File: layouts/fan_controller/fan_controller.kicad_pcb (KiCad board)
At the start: 2 copper layers, 6 parts

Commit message: Add MCU as build target
use this ato branch to fix build:
https://github.com/atopile/atopile/pull/979
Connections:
- D1 pad 2: gnd-2 -> gnd-1
- FanConnector1 pad 1: gnd-2 -> gnd-1
- Q1 pad 2: gnd-2 -> gnd-1
- Q1 pad 3: gnd -> gnd-2
- R1 pad 2: gnd-1 -> gnd
- R2 pad 2: gnd-2 -> gnd-1
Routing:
- net gnd-2: track 6.53 -> 0.00 mm
- net gnd-1: track 0.00 -> 6.53 mm

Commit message: Migrate layout partially
omit routing and zones amongst others
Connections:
- D1 pad 2: gnd-1 -> gnd
- FanConnector1 pad 1: gnd-1 -> gnd
- Q1 pad 2: gnd-1 -> gnd
- Q1 pad 3: gnd-2 -> gnd-1
- R1 pad 2: gnd -> gnd-2
- R2 pad 2: gnd-1 -> gnd
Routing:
- net gnd-1: track 6.53 -> 0.00 mm
- net gnd: track 0.00 -> 6.53 mm
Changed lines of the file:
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@@
             (outputdirectory "")))
     (net 0 "")
-    (net 1 "gnd-1")
-    (net 2 "gnd-2")
+    (net 1 "gnd")
+    (net 2 "gnd-1")
     (net 3 "cathode")
     (net 4 "fan_connector.footprint.pins[3].net-net")
     (net 5 "hv")
-    (net 6 "gnd")
+    (net 6 "gnd-2")
     (net 7 "line")
     (net 8 "fan_connector.footprint.pins[2].net-net")
@@
             (layers "F.Cu" "F.Paste" "F.Mask")
             (remove_unused_layers no)
-            (net 1 "gnd-1")))
+            (net 1 "gnd")))
     (footprint "atopile:SOT-23-3_L2.9-W1.3-P1.90-LS2.4-BL-1-fcaf94"
         (layer "F.Cu")
@@
             (layers "F.Cu" "F.Paste" "F.Mask")
             (remove_unused_layers no)
-            (net 1 "gnd-1"))
+            (net 1 "gnd"))
         (pad "3" smd rect
             (at 0 -1 0)
@@
             (layers "F.Cu" "F.Paste" "F.Mask")
             (remove_unused_layers no)
-            (net 2 "gnd-2")))
+            (net 2 "gnd-1")))
     (footprint "atopile:R0603-ebcab9"
         (layer "F.Cu")
@@
             (layers "F.Cu" "F.Paste" "F.Mask")
             (remove_unused_layers no)
-            (net 6 "gnd")))
+            (net 6 "gnd-2")))
     (footprint "atopile:CONN-SMD_1.25-2P-ea2134"
         (layer "F.Cu")
@@
             (layers "F.Cu" "F.Paste" "F.Mask")
             (remove_unused_layers no)
-            (net 1 "gnd-1"))
+            (net 1 "gnd"))
         (pad "2" smd rect
             (at 0.63 -1.45 90)
@@
             (layers "F.Cu" "F.Paste" "F.Mask")
             (remove_unused_layers no)
-            (net 1 "gnd-1")))
+            (net 1 "gnd")))
     (segment
         (start 10.83 -4.5)

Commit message: Update layouts
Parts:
- D2: value infV -> (none)
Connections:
- Q1 pad 3: gnd-1 -> gnd-2
- R1 pad 2: gnd-2 -> gnd-1

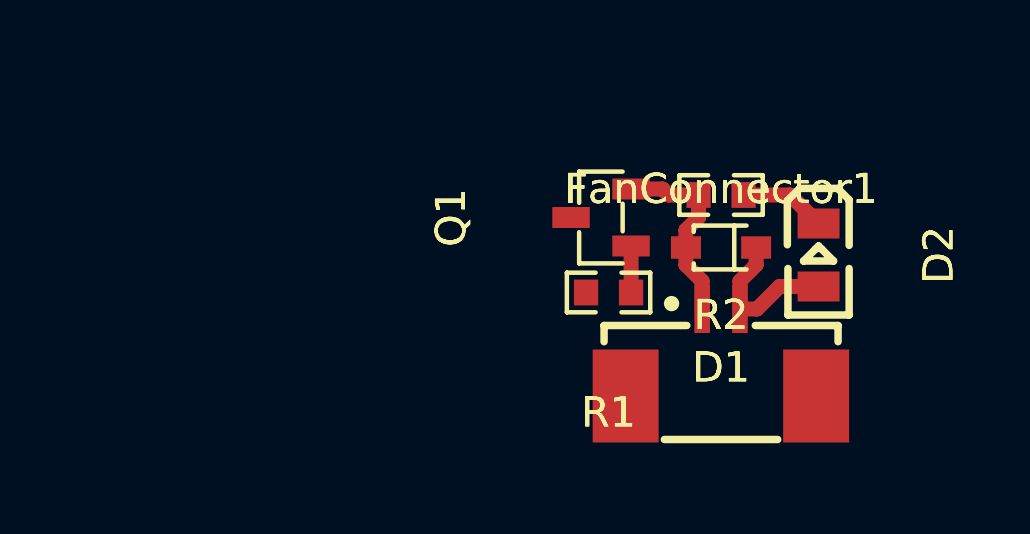
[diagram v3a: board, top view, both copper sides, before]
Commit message: Update layout
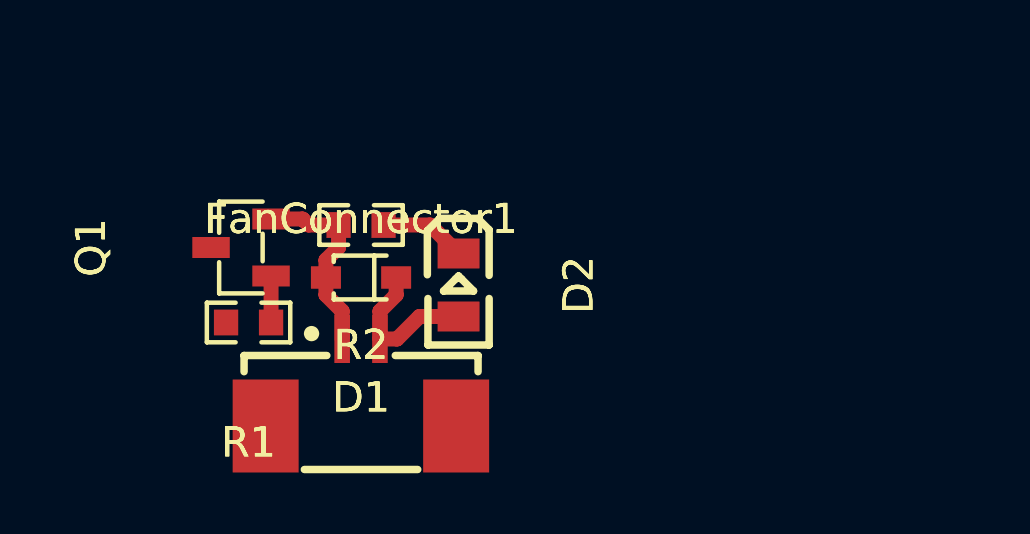
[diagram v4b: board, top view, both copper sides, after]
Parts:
- moved D1 12.0 mm to (0.00, -3.50)
- moved D2 12.0 mm to (3.25, -3.25)
- moved FanConnector1 12.0 mm to (0.00, 0.00)
- moved Q1 12.0 mm to (-4.00, -4.50)
- moved R1 12.0 mm to (-3.75, -2.00)
- moved R2 12.0 mm to (0.00, -5.25)

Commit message: do some layouts
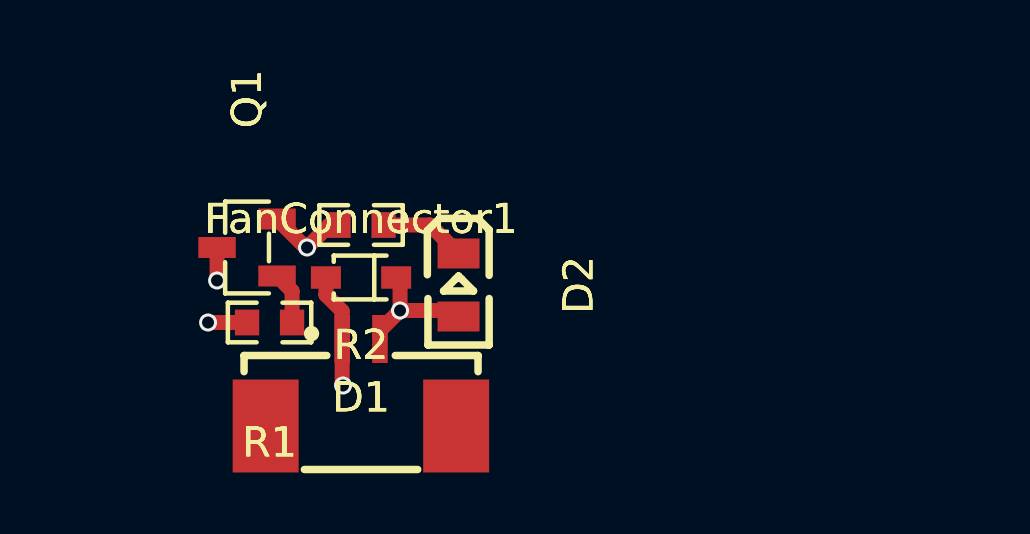
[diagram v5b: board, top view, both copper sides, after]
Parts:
- Q1: footprint atopile:SOT-23-3_L2.9-W1.3-P1.90-LS2.4-BL-1-fcaf94 -> atopile:SOT-23-3_L2.9-W1.3-P1.90-LS2.4-BR-688f29
- moved R1 0.70 mm to (-3.05, -2.00)
- moved Q1 0.20 mm to (-3.80, -4.50), turned to 0 degrees
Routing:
- net gnd-1: track 0.00 -> 1.30 mm, vias 0 -> 1
- net gnd-2: track 0.00 -> 1.10 mm, vias 0 -> 1
- net hv: track 5.20 -> 4.41 mm, vias 0 -> 1
- net gnd: track 6.53 -> 6.66 mm, vias 0 -> 2

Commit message: Try to fix fuses
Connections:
- Q1 pad 3: gnd-2 -> gnd-1
- R1 pad 2: gnd-1 -> gnd-2
